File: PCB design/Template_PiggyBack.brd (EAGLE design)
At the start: 63.5 x 88.6 mm, 46 parts, among them CN1 USB power supply, IC1 MCP6002, IC3 MCP6002, IC4 REG1117

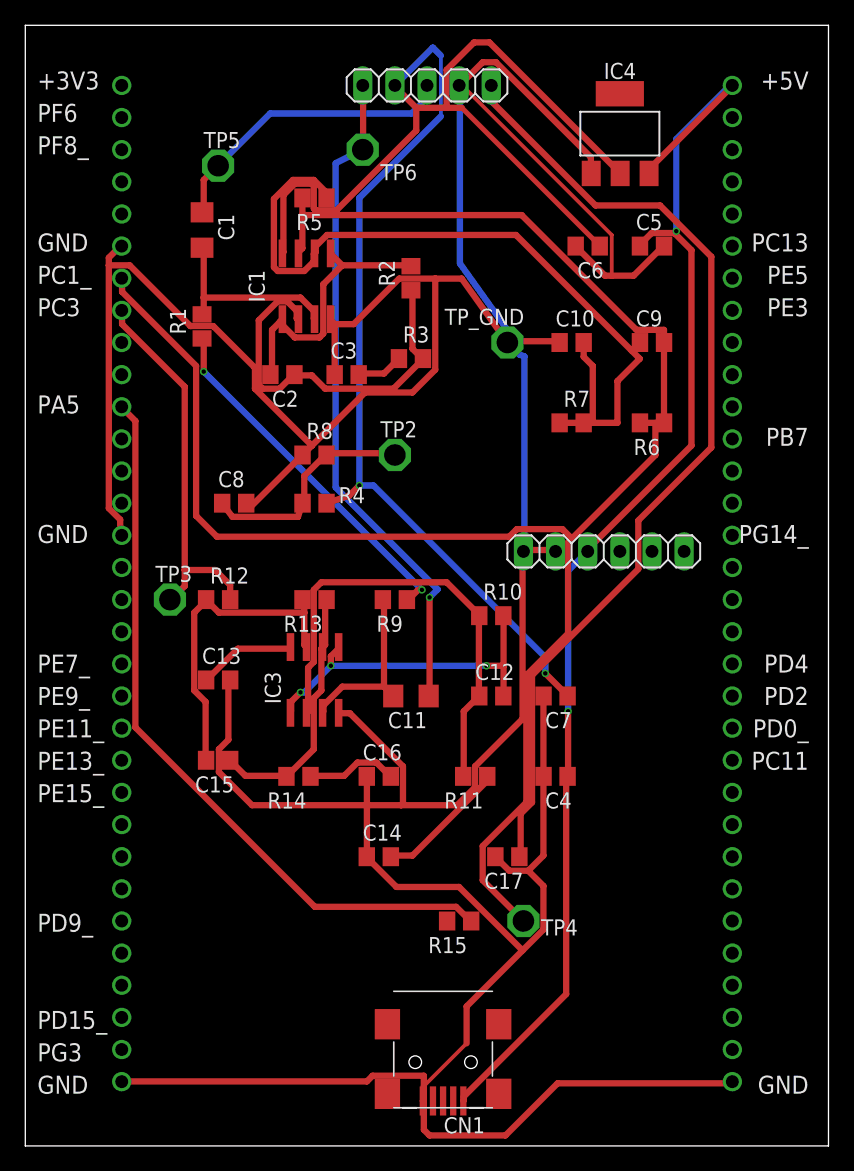
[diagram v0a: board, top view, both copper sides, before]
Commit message: layout mission complete
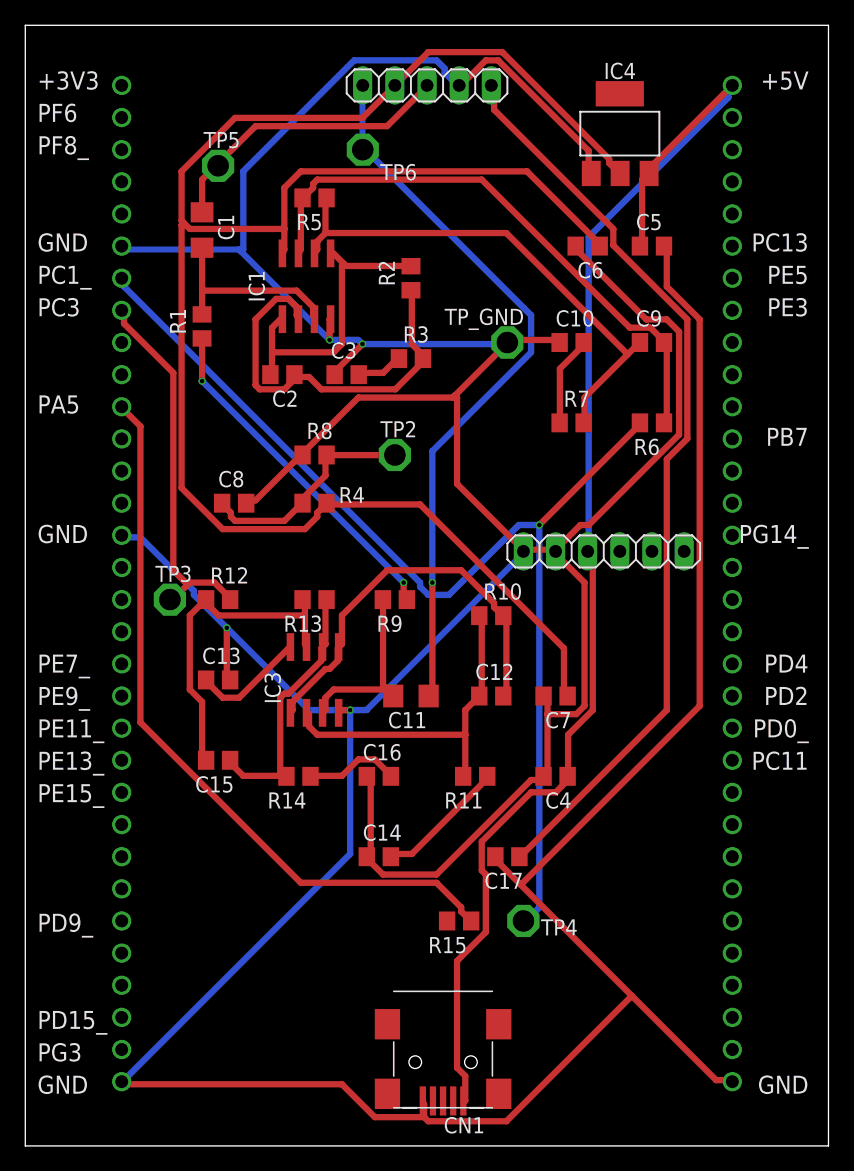
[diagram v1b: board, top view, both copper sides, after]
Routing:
- net GND: track 361.2 -> 426.9 mm, vias 0 -> 4
- net +3V3: track 134.2 -> 150.6 mm, vias 2 -> 0
- net N$8: track 55.3 -> 40.8 mm
- net N$9: track 37.7 -> 27.2 mm
- net PC1_: track 99.7 -> 89.5 mm, vias 0 -> 1
- net N$12: track 26.9 -> 32.0 mm, vias 3 -> 0
- net VCO: track 77.4 -> 72.9 mm
- net +5V: track 103.2 -> 107.4 mm, vias 2 -> 0
- net IF_Q: track 53.2 -> 57.3 mm
- net N$3: track 9.27 -> 7.18 mm
- net N$5: track 22.0 -> 23.8 mm
- net N$7: track 44.2 -> 45.9 mm
- net N$2: track 30.6 -> 31.9 mm
- net VCC: track 7.74 -> 8.95 mm
- net V_GND: track 28.6 -> 27.5 mm
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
